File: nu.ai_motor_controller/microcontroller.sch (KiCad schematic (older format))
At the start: 41 parts, among them J10 Conn_02x05_Odd_Even, J11 DX4R105JJCR1800, J9 Conn_02x12_Odd_Even, SW1 TACTILE_SWITCH, U9 ATmega32U4-AU, Y1 7M-16.000MAAE-T

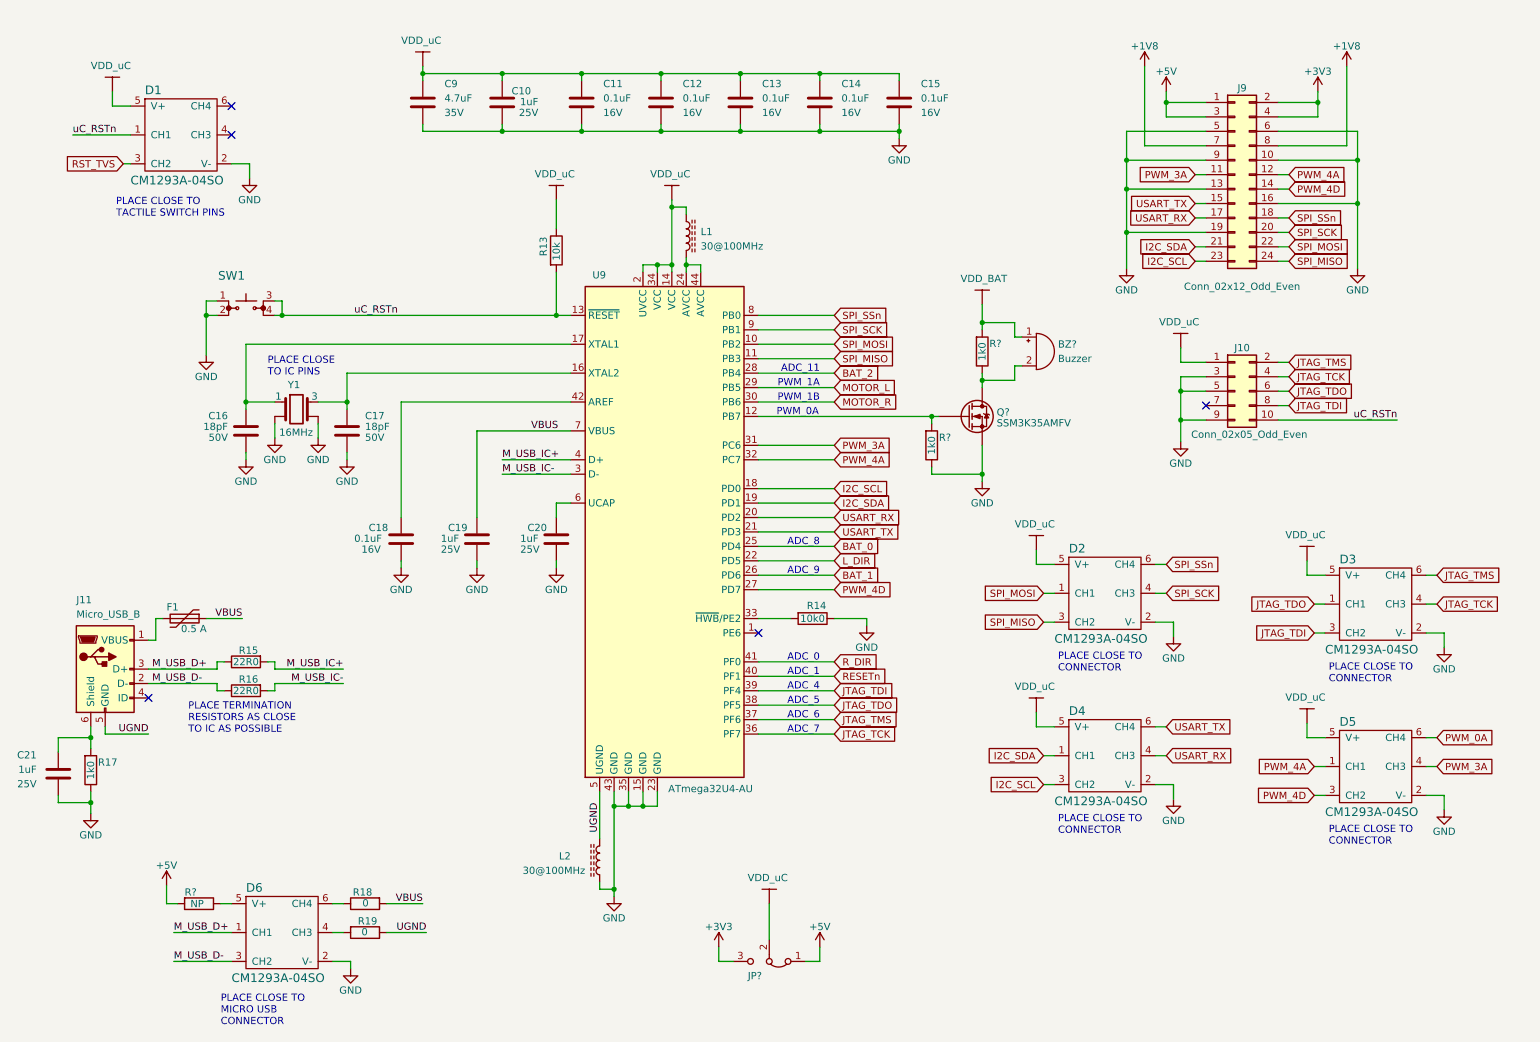
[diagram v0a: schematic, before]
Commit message: automated commit
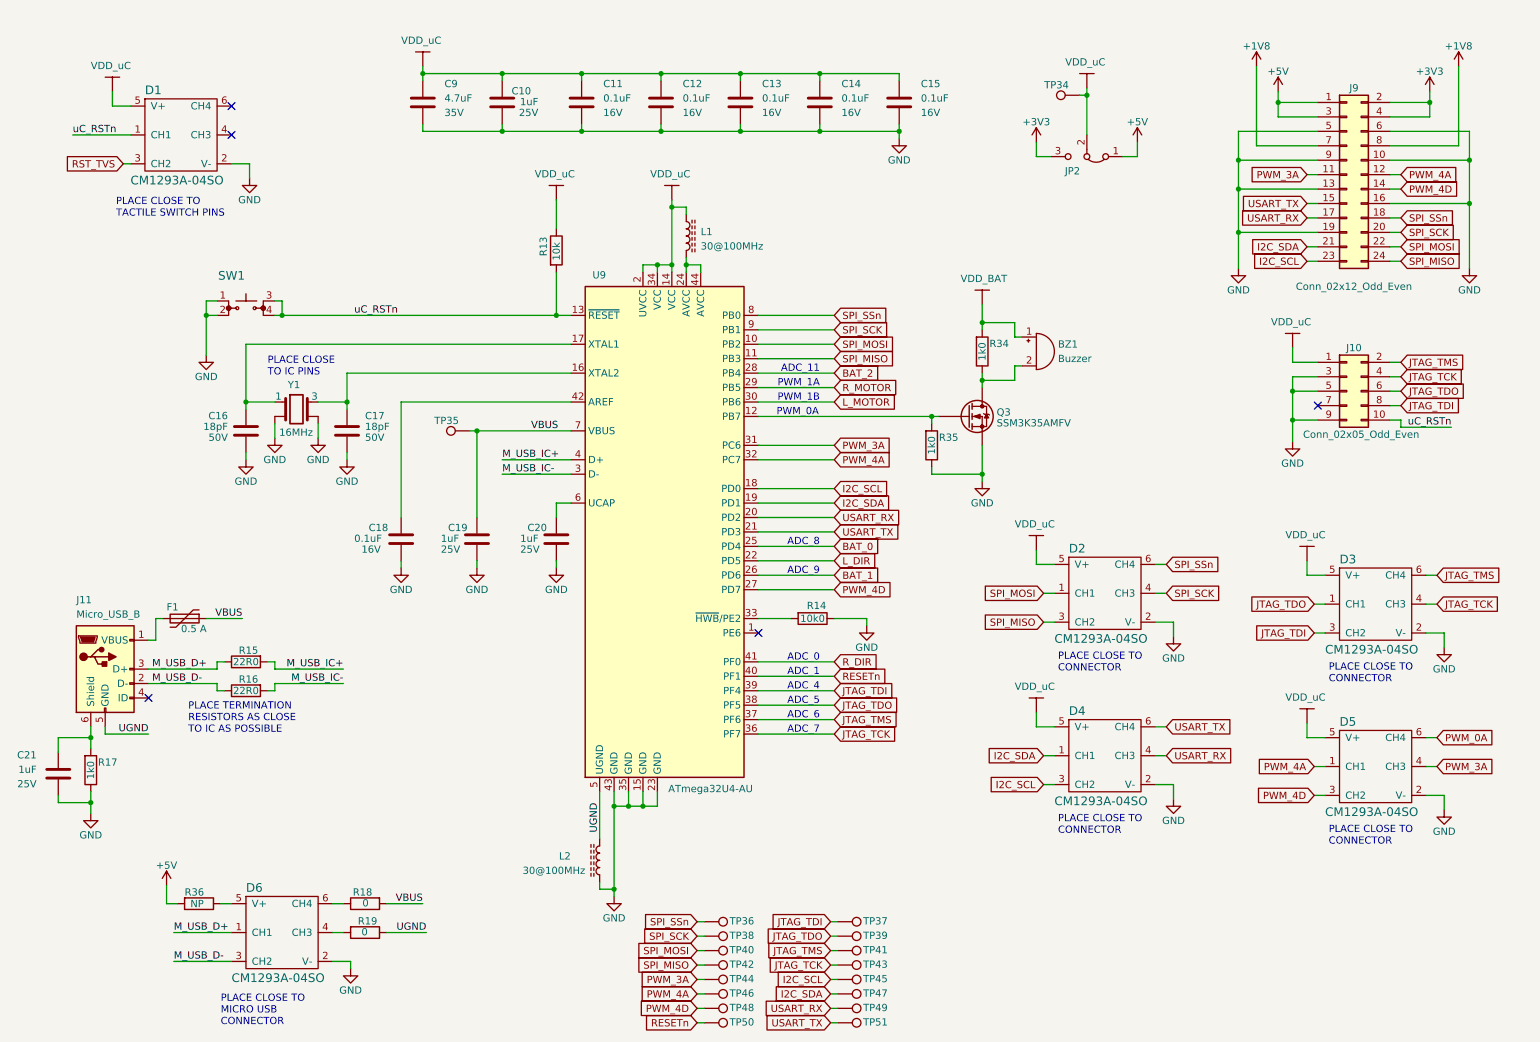
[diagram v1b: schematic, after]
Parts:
- added TP34, TP35, TP36, TP37, TP38, TP39, TP40, TP41, TP42, TP43, TP44, TP45, TP46, TP47, TP48, TP49, TP50, TP51: PTH_0.5_mm, symbol custom:PTH_0.5_mm
- gave numbers to parts that had none: 6
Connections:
- net I2C_SCL: now also TP45.1
- net I2C_SDA: now also TP47.1
- net JTAG_TCK: now also TP43.1
- net JTAG_TDI: now also TP37.1
- net JTAG_TDO: now also TP39.1
- net JTAG_TMS: now also TP41.1
- net PWM_3A: now also TP44.1
- net PWM_4A: now also TP46.1
- net PWM_4D: now also TP48.1
- net RESETn: now also TP50.1
- net SPI_MISO: now also TP42.1
- net SPI_MOSI: now also TP40.1
- net SPI_SCK: now also TP38.1
- net SPI_SSn: now also TP36.1
- net USART_RX: now also TP49.1
- net USART_TX: now also TP51.1
- net VBUS: now also TP35.1
- net VDD_uC: now also TP34.1
- net MOTOR_L renamed R_MOTOR
- net MOTOR_R renamed L_MOTOR
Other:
- moved on the sheet: J10, J9, JP2

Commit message: automated commit
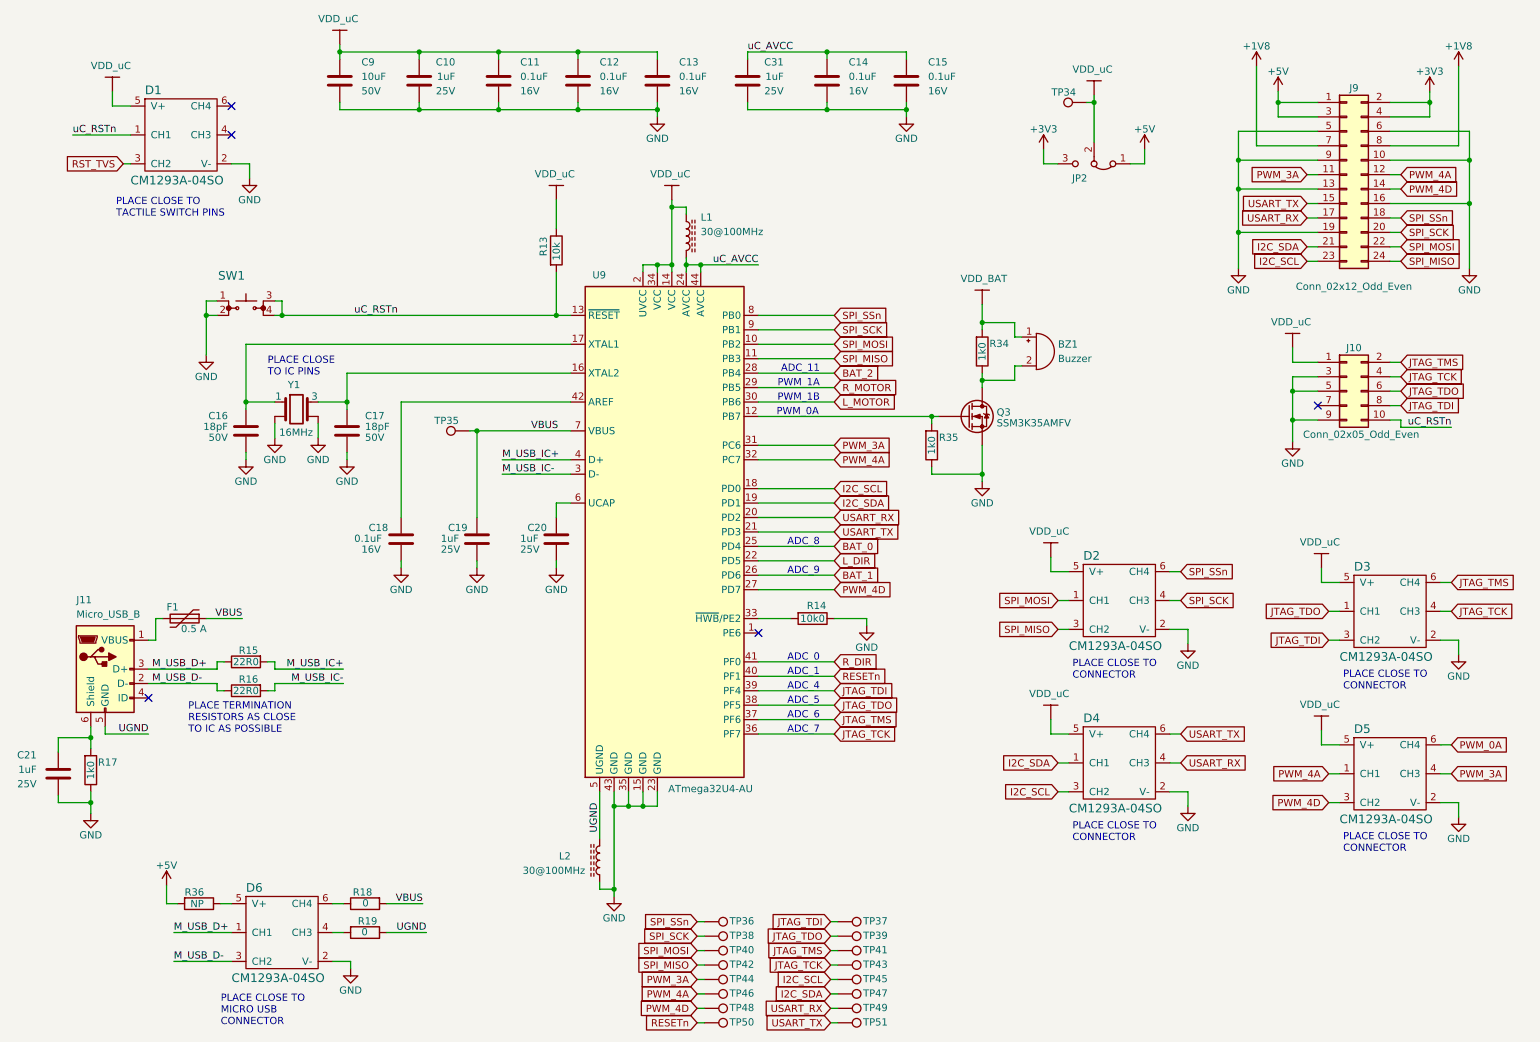
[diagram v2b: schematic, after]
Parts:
- removed C9: ‎CL21A475KLCLQNC‎, Capacitor_SMD:C_0805_2012Metric, symbol custom:‎CL21A475KLCLQNC‎
- added C31: CL10B105KA8NNNC, Capacitor_SMD:C_0603_1608Metric, symbol custom:CL10B105KA8NNNC
- added C9: CL10B103KB8SFNC, Capacitor_SMD:C_0603_1608Metric, symbol custom:CL10B103KB8SFNC
- BZ1: footprint (none) -> custom:0.5_IN_BUZZER
- D1, D2, D3, D4, D5, D6: footprint SOT-457 -> custom:SOT-457
- J10: footprint (none) -> Connector_PinHeader_2.54mm:PinHeader_2x05_P2.54mm_Vertical
- J9: footprint (none) -> Connector_PinHeader_2.54mm:PinHeader_2x12_P2.54mm_Vertical
- JP2: footprint (none) -> Connector_PinHeader_2.54mm:PinHeader_1x03_P2.54mm_Vertical
- L1, L2: footprint 0603 -> Inductor_SMD:L_0603_1608Metric
- R13, R14, R15, R16, R17, R34, R35: footprint 0603 -> Resistor_SMD:R_0603_1608Metric
- R36: footprint 0603 -> custom:NP_0603
- TP34, TP35, TP36, TP37, TP38, TP39, TP40, TP41, TP42, TP43, TP44, TP45, TP46, TP47, TP48, TP49, TP50, TP51: footprint (none) -> TestPoint:TestPoint_THTPad_D1.0mm_Drill0.5mm
- Y1: footprint (none) -> Crystal:Crystal_SMD_3225-4Pin_3.2x2.5mm
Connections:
- net GND: now also C31.2, C9.2
- net VDD_uC: now also C9.1; no longer C14.1, C15.1
- net uC_AVCC: now reaches L1.2, U9.24 (AVCC), U9.44 (AVCC)
- net uC_AVCC: now also C14.1, C15.1, C31.1
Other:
- moved on the sheet: C10, C11, C12, C13, C14, C15, D2, D3, D4, D5, JP2, TP34

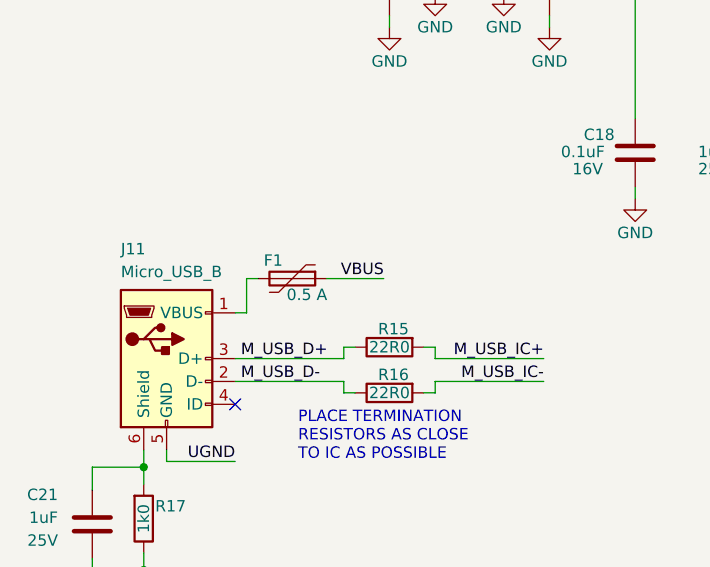
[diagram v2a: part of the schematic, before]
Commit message: automated commit
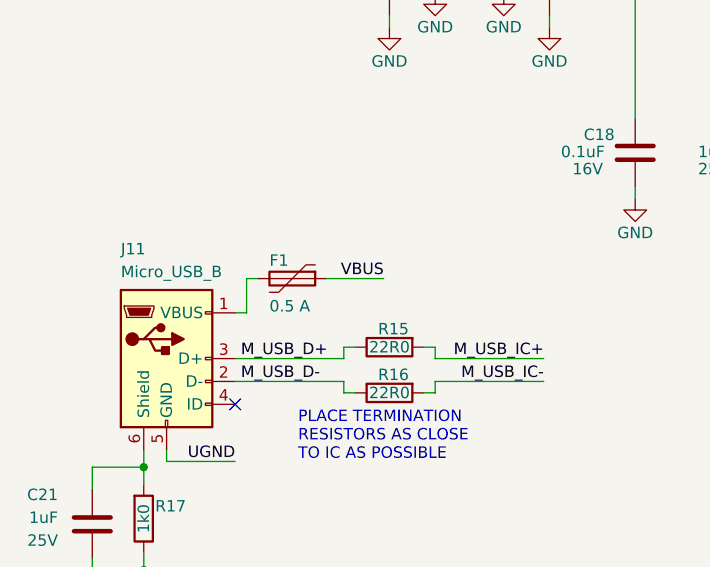
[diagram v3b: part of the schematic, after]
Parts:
- F1: footprint 1812 -> custom:MF-MSMF050-2
- J11: footprint (none) -> custom:DX4R105JJCR1800‎_MICRO_USB_B_CONNECTOR
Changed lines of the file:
@@
 F 0 "J11" H 1125 5525 50  0000 L BNN
 F 1 "DX4R105JJCR1800" H 1025 4275 50  0001 L BNN
-F 2 "" H 1475 5025 50  0001 C CNN
+F 2 "custom:DX4R105JJCR1800‎_MICRO_USB_B_CONNECTOR" H 1475 5025 50  0001 C CNN
 F 3 "SJ113218.pdf" H 1475 5025 50  0001 L BNN
 F 4 "Micro_USB_B" H 1125 5425 50  0000 L BNN "Description"
@@
 Text Label 2975 5175 2    50   ~ 0
 M_USB_IC-
-$Comp
-L custom:MF-MSMF050-2 F1
-U 1 1 5C440655
-P 1875 4725
-F 0 "F1" V 1825 4600 50  0000 L BNN
-F 1 "MF-MSMF050-2" H 1775 4200 50  0001 L BNN
-F 2 "1812" H 1775 4275 50  0001 L BNN
-F 3 "~/datasheets/mfmsmf.pdf" H 1775 4100 50  0001 L BNN
-F 4 "0.5 A" V 1975 4700 50  0000 L BNN "Rating"
-	1    1875 4725
-	0    1    1    0
-$EndComp
 Wire Wire Line
 	2025 4725 2275 4725
@@
 uC_AVCC
 Connection ~ 5150 1200
+$Comp
+L custom:MF-MSMF050-2 F1
+U 1 1 5C5A71F2
+P 1875 4725
+F 0 "F1" V 1825 4625 50  0000 L BNN
+F 1 "MF-MSMF050-2" H 1775 4200 50  0001 L BNN
+F 2 "custom:MF-MSMF050-2" H 1775 4275 50  0001 L BNN
+F 3 "/home/dj/datasheets/mfmsmf.pdf" H 1775 4100 50  0001 L BNN
+F 4 "0.5 A" V 2025 4625 50  0000 L BNN "Rating"
+	1    1875 4725
+	0    1    1    0
+$EndComp
 $EndSCHEMATC
